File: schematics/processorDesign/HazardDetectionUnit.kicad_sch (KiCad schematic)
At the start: 9 parts

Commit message: the interrupt is now working correctly
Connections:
- net at U?.: now also U?.4
- net at U?.: now also U?.3
- net at U?.: now also U?.1
- net at U?.: now also U?.2

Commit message: the processor is now up and running , tested and verified , except for the part related to labels due to a bug in the assembler
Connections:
- net at U?.: now also U?.4
- net at U?.: now also U?.3
- net at U?.: now also U?.1
- net at U?.: now also U?.2

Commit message: the processor is now up and running , tested and verified completly for almost most of the things
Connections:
- net at U?.: now also U?.4
- net at U?.: now also U?.3
- net at U?.: now also U?.1
- net at U?.: now also U?.2

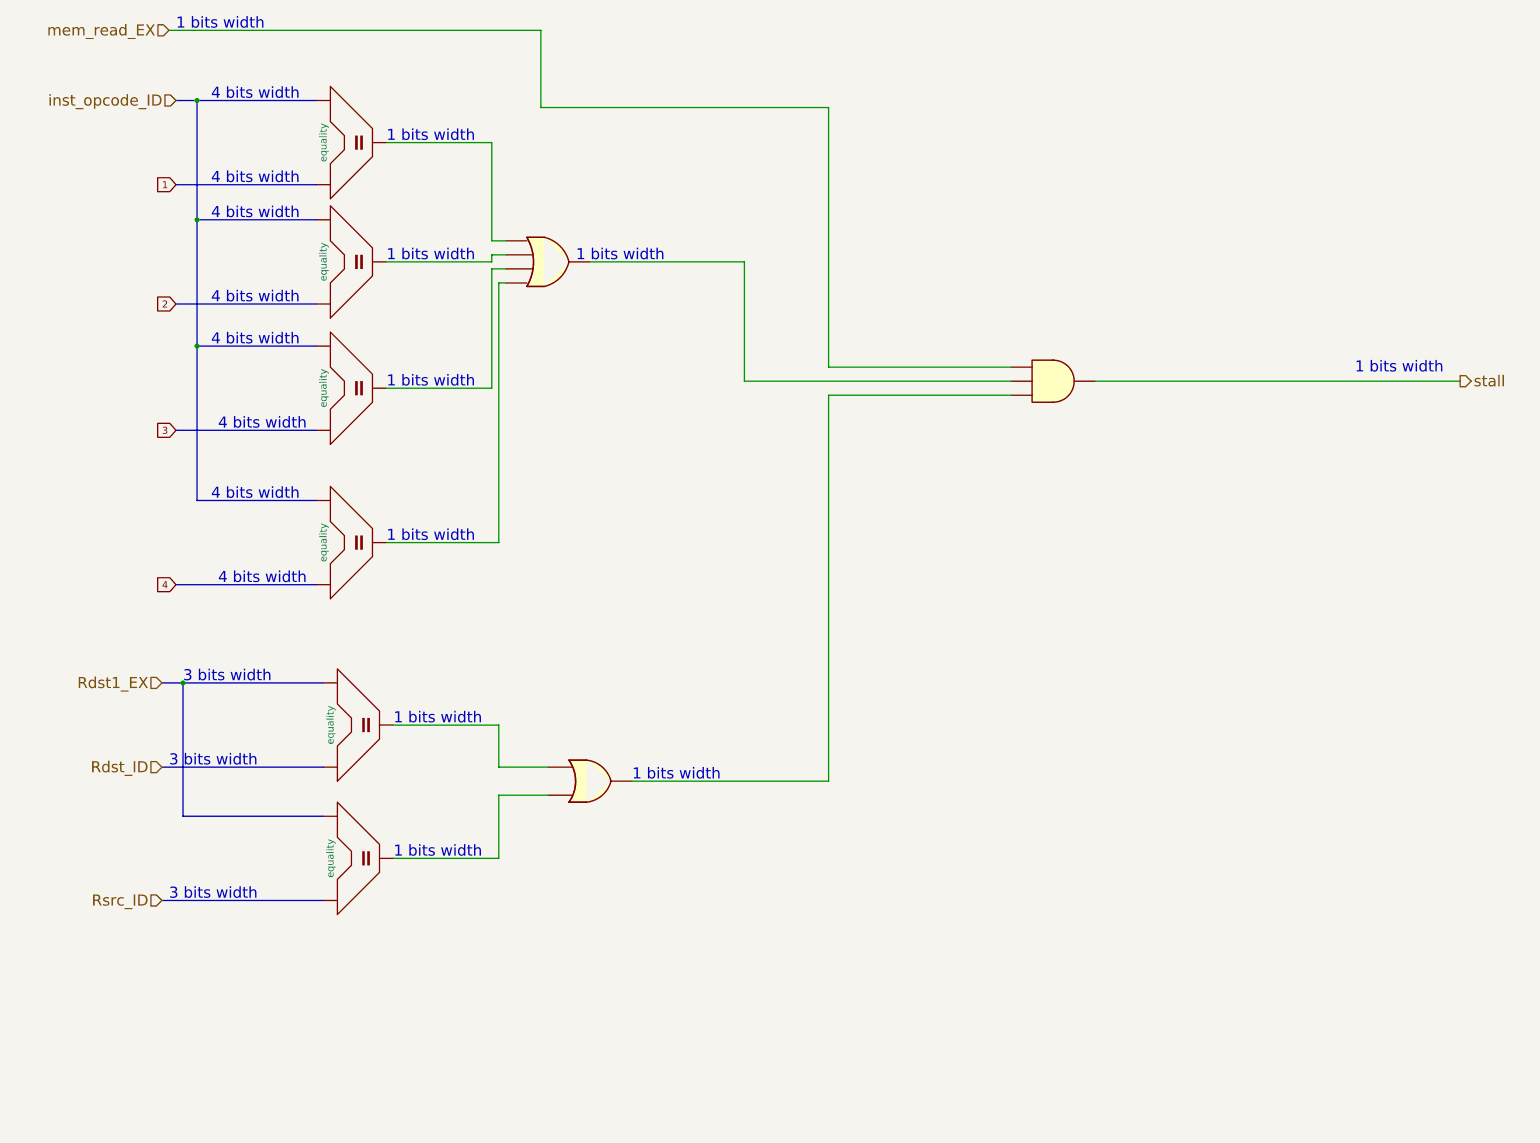
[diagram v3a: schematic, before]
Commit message: added small code to EDU
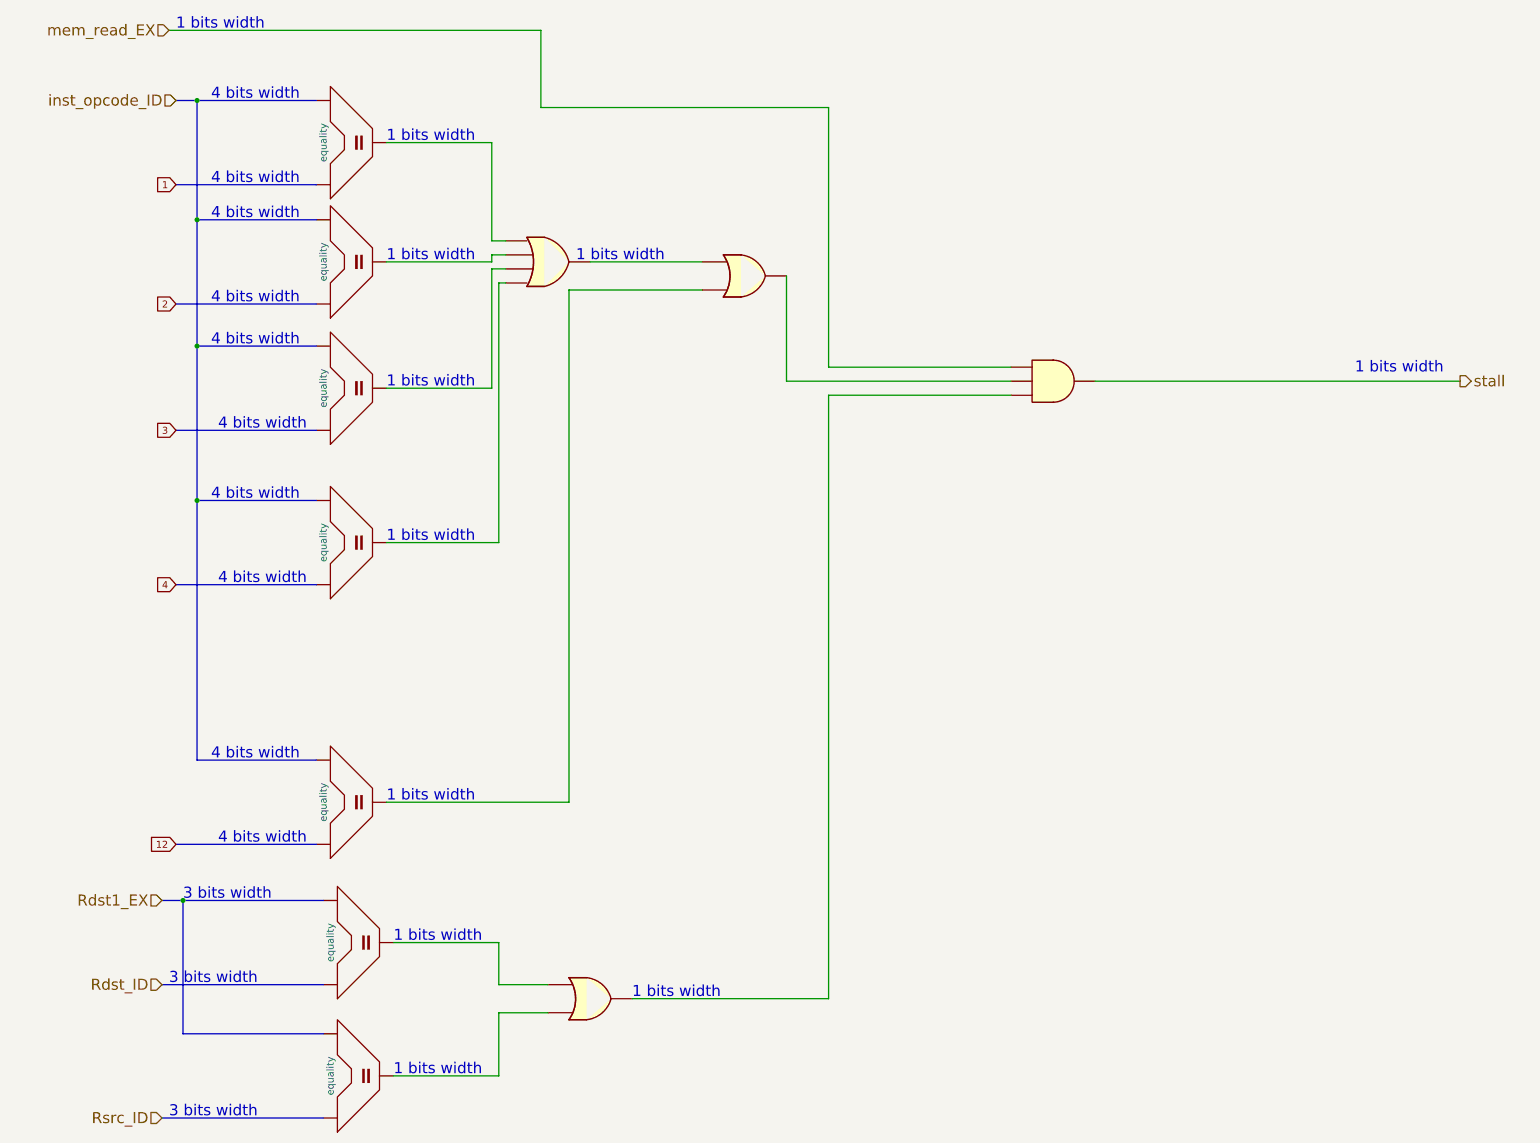
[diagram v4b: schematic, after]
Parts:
- added U?: 4071, symbol 4xxx:4071
- added U?: equality, symbol computerArchProj:equality
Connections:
- net at U?.: now also U?.4
- net at U?.: now also U?.3
- net at U?.: now also U?.1
- net at U?.1: now also U?.1; no longer U?.2
- net at U?.: now also U?.2
- new net: U?., U?.2
- new net: U?.2, U?.3
